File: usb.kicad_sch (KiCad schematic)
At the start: 7 parts, among them J2 TYPE-C 16PIN 2MD(073), U4 USBLC6-2P6, U5 USBLC6-2P6

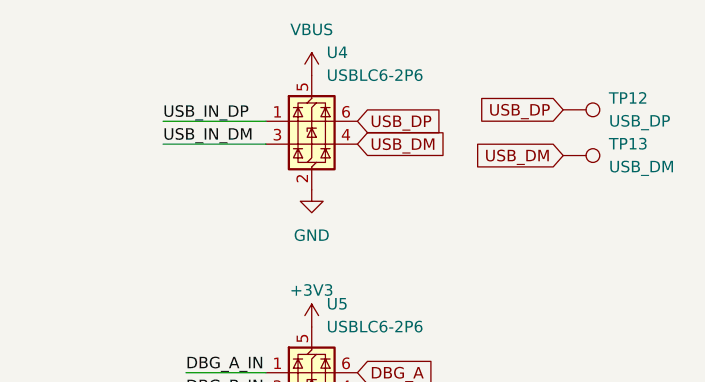
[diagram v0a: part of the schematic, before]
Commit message: final review, fixes, cleanup
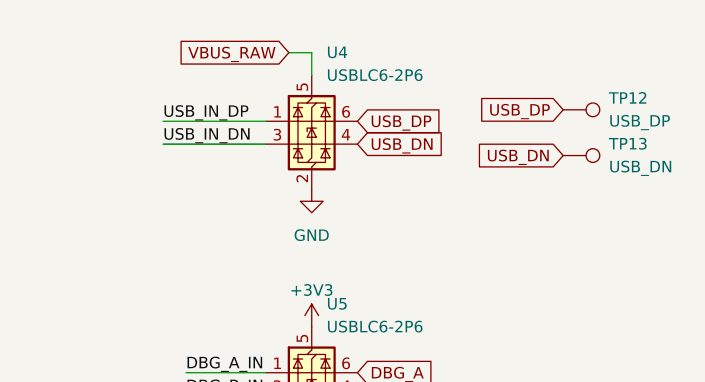
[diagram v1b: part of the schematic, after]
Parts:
- TP13: value USB_DM -> USB_DN
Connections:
- net USB_IN_DM is gone; now on net USB_IN_DN: U4.3 (I/O2)
- net VBUS is gone; now on net VBUS_RAW: U4.5 (VBUS)
- net USB_DM renamed USB_DN
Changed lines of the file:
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@@
+	(wire
+		(pts
+			(xy 181.61 78.74) (xy 184.15 78.74)
+		)
+		(stroke
+			(width 0)
+			(type default)
+		)
+	)
 	(wire
 		(pts
@@
 		(pts
 			(xy 104.14 111.76) (xy 118.11 111.76)
+		)
+		(stroke
+			(width 0)
+			(type default)
+		)
+	)
+	(wire
+		(pts
+			(xy 184.15 78.74) (xy 184.15 81.28)
 		)
 		(stroke
@@
 		)
 	)
-	(label "USB_IN_DM"
+	(label "USB_IN_DN"
 		(at 167.64 88.9 0)
 		(effects
@@
 		)
 	)
-	(global_label "USB_DM"
+	(global_label "USB_DN"
 		(shape input)
 		(at 212.09 90.17 180)
@@
 		)
 		(property "Intersheetrefs" "${INTERSHEET_REFS}"
-			(at 201.6058 90.17 0)
+			(at 201.7267 90.17 0)
 			(effects
 				(font
@@
 		)
 	)
+	(global_label "VBUS_RAW"
+		(shape input)
+		(at 181.61 78.74 180)
+		(fields_autoplaced yes)
+		(effects
+			(font
+				(size 1.27 1.27)
+			)
+			(justify right)
+		)
+		(property "Intersheetrefs" "${INTERSHEET_REFS}"
+			(at 168.9486 78.74 0)
+			(effects
+				(font
+					(size 1.27 1.27)
+				)
+				(justify right)
+				(hide yes)
+			)
+		)
+	)
 	(global_label "DBG_B"
 		(shape input)
@@
 		)
 	)
-	(global_label "USB_DM"
+	(global_label "USB_DN"
 		(shape input)
 		(at 189.23 88.9 0)
@@
 		)
 		(property "Intersheetrefs" "${INTERSHEET_REFS}"
-			(at 199.7142 88.9 0)
+			(at 199.5933 88.9 0)
 			(effects
 				(font
@@
 	)
 	(symbol
-		(lib_id "power:VBUS")
-		(at 184.15 81.28 0)
-		(unit 1)
-		(exclude_from_sim no)
-		(in_bom yes)
-		(on_board yes)
-		(dnp no)
-		(fields_autoplaced yes)
-		(property "Reference" "#PWR048"
-			(at 184.15 85.09 0)
-			(effects
-				(font
-					(size 1.27 1.27)
-				)
-				(hide yes)
-			)
-		)
-		(property "Value" "VBUS"
-			(at 184.15 76.2 0)
-			(effects
-				(font
-					(size 1.27 1.27)
-				)
-			)
-		)
-		(property "Footprint" ""
-			(at 184.15 81.28 0)
-			(effects
-				(font
-					(size 1.27 1.27)
-				)
-				(hide yes)
-			)
-		)
-		(property "Datasheet" ""
-			(at 184.15 81.28 0)
-			(effects
-				(font
-					(size 1.27 1.27)
-				)
-				(hide yes)
-			)
-		)
-		(property "Description" "Power symbol creates a global label with name \"VBUS\""
-			(at 184.15 81.28 0)
-			(effects
-				(font
-					(size 1.27 1.27)
-				)
-				(hide yes)
-			)
-		)
-		(pin "1"
-		)
-		(instances
-			(project "rc_keychain"
-				(path "/c6cb5a1d-9f97-4766-8582-a9e93ed049e4/69f5d0af-289d-4671-84fe-e5e630f97c44"
-					(reference "#PWR048")
-					(unit 1)
-				)
-			)
-		)
-	)
-	(symbol
 		(lib_id "power:GND")
 		(at 96.52 99.06 0)
@@
 			)
 		)
-		(property "Value" "USB_DM"
+		(property "Value" "USB_DN"
 			(at 217.17 91.4399 90)
 			(effects
